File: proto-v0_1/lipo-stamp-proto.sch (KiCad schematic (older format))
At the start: 27 parts, among them Q1 Q_PMOS_GSD, U3 MCP73832-2-OT, U4 AP2112K-3.3, U5 AP9101CK6, U6 FS8205

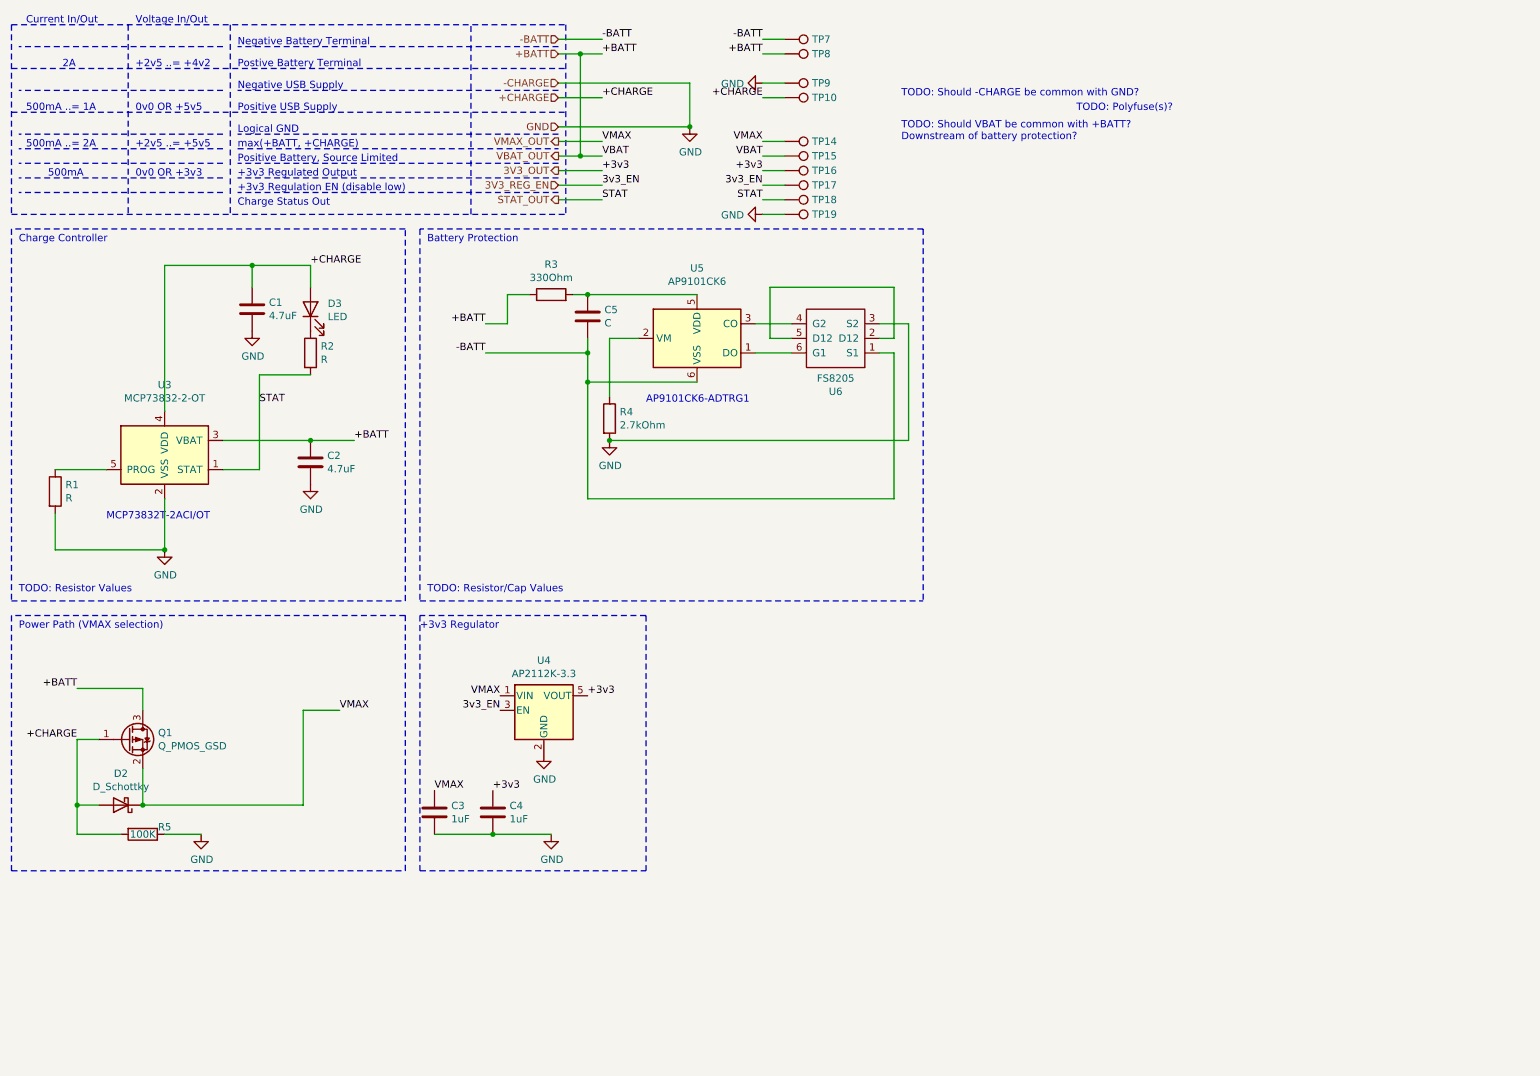
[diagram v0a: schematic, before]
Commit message: Going to start routing
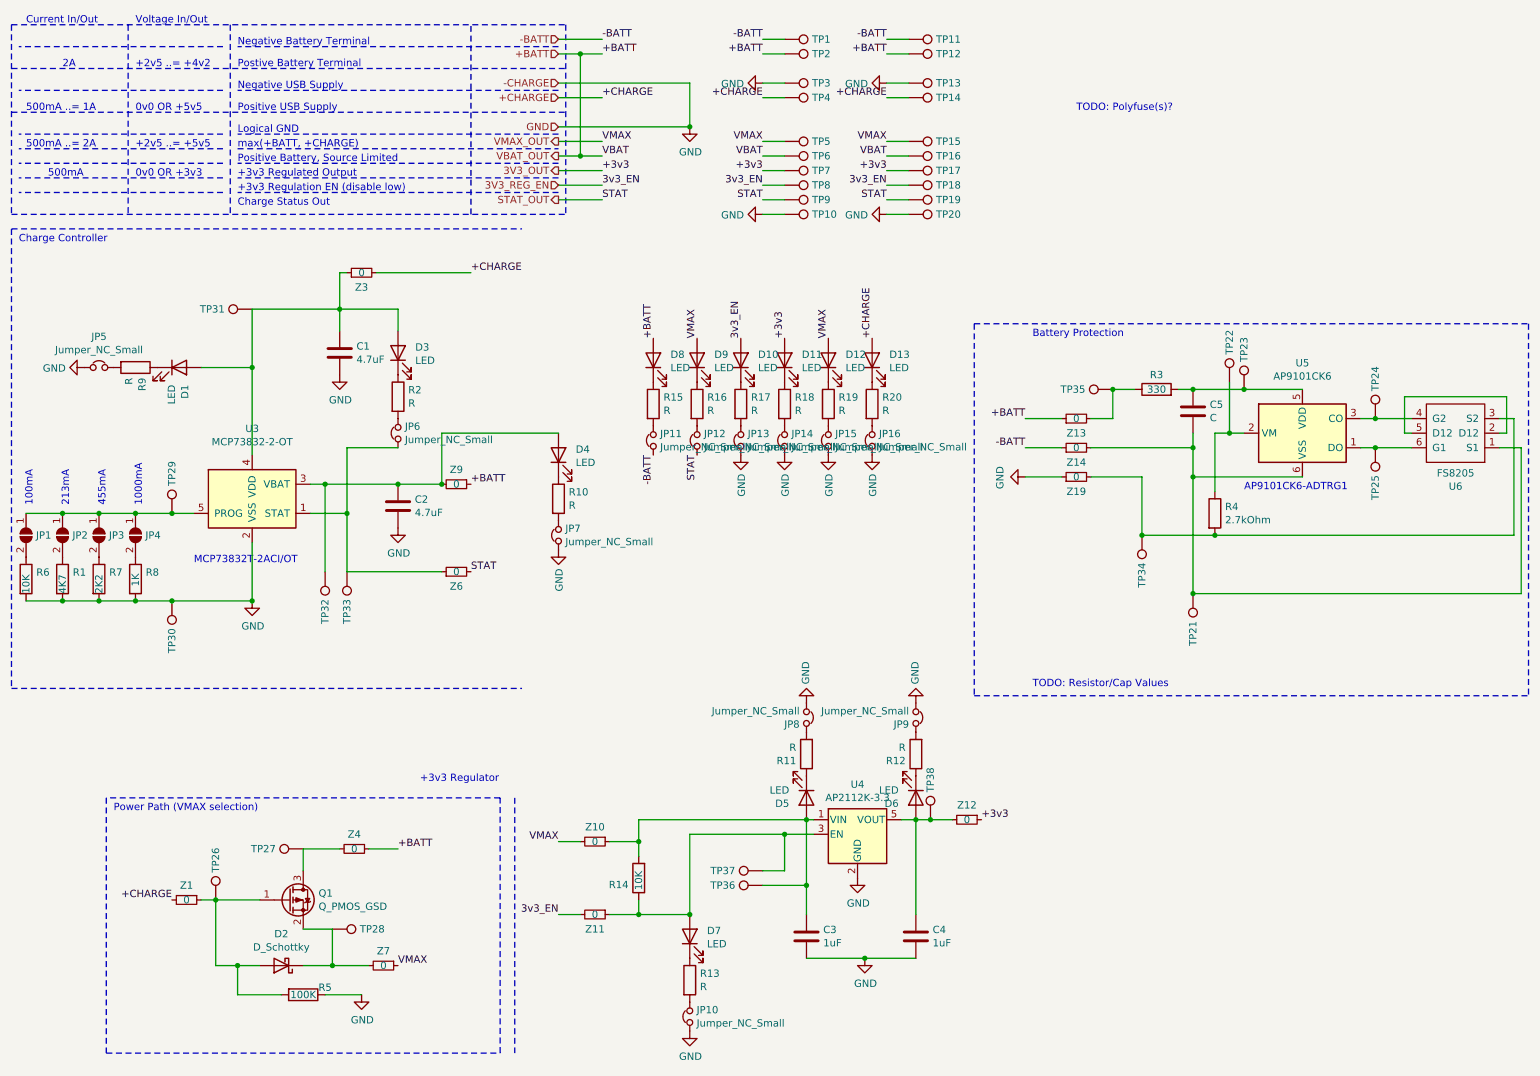
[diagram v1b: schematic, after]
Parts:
- added D1, D10, D11, D12, D13, D4, D5, D6, D7, D8, D9: LED, LED_SMD:LED_0805_2012Metric, symbol Device:LED
- added JP1, JP2, JP3, JP4: SolderJumper_2_Open, Jumper:SolderJumper-2_P1.3mm_Open_TrianglePad1.0x1.5mm, symbol Jumper:SolderJumper_2_Open
- added JP10, JP11, JP12, JP13, JP14, JP15, JP16, JP5, JP6, JP7, JP8, JP9: Jumper_NC_Small, Jumper:SolderJumper-2_P1.3mm_Bridged_RoundedPad1.0x1.5mm, symbol Device:Jumper_NC_Small
- added R10, R11, R12, R13, R15, R16, R17, R18, R19, R20, R9: R, Resistor_SMD:R_0805_2012Metric, symbol Device:R
- added R14, R6: 10K, Resistor_SMD:R_0805_2012Metric, symbol Device:R
- added R7: 2K2, Resistor_SMD:R_0805_2012Metric, symbol Device:R
- added R8: 1K, Resistor_SMD:R_0805_2012Metric, symbol Device:R
- added TP1, TP11, TP12, TP13, TP2, TP20, TP21, TP22, TP23, TP24, TP25, TP26, TP27, TP28, TP29, TP3, TP30, TP31, TP32, TP33, TP34, TP35, TP36, TP37, TP38, TP4, TP5, TP6: TestPoint, Everything:castellated-2-pin, symbol Connector:TestPoint
- added Z1, Z10, Z11, Z12, Z13, Z14, Z19, Z3, Z4, Z6, Z7, Z9: 0, Resistor_SMD:R_0805_2012Metric, symbol Device:R_Small
- R1: value R -> 4K7
- R3: value 330Ohm -> 330
- TP10, TP14, TP15, TP16, TP17, TP18, TP19, TP7, TP8, TP9: footprint Connector_PinHeader_2.54mm:PinHeader_1x01_P2.54mm_Vertical -> Everything:castellated-2-pin
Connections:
- net +BATT: now also TP16.1, D8.2 (A), TP12.1, TP2.1, TP6.1, Z13.1, Z4.1, Z9.1; no longer C2.1, Q1.3 (D), R3.1, TP15.1, TP8.1, U3.3 (VBAT)
- net +CHARGE: now also TP14.1, D13.2 (A), TP4.1, Z1.2, Z3.2; no longer C1.1, D2.2 (A), D3.2 (A), Q1.1 (G), R5.2, TP10.1, U3.4 (VDD)
- net -BATT: now also JP11.1, TP1.1, TP11.1, Z14.1; no longer C5.2, TP7.1, U5.6 (VSS), U6.1 (S1)
- net 3V3_OUT: now also TP17.1, TP7.1, D11.2 (A), Z12.1; no longer C4.1, TP16.1, U4.5 (VOUT)
- net 3V3_REG_EN: now also TP18.1, TP8.1, D10.2 (A), Z11.2; no longer TP17.1, U4.3 (EN)
- net GND: now also TP10.1, JP10.1, JP13.1, JP14.1, JP15.1, JP16.1, JP5.1, JP7.1, JP8.1, JP9.1, R6.2, R7.2, R8.2, TP13.1, TP20.1, TP3.1, TP30.1, Z19.1; no longer R4.2, TP19.1, TP9.1, U6.3 (S2)
- net STAT_OUT: now also TP19.1, TP9.1, JP12.1, Z6.2; no longer R2.2, TP18.1, U3.1 (STAT)
- net VMAX_OUT: now also TP15.1, D12.2 (A), D9.2 (A), TP5.1, Z10.2, Z7.1; no longer C3.1, D2.1 (K), Q1.2 (S), TP14.1, U4.1 (VIN)
- net at C5.1, R3.2, U5.5 (VDD): now also TP23.1
- net at R4.1, U5.2 (VM): now also TP22.1
- net at U3.5 (PROG): now also JP1.1 (A), JP2.1 (A), JP3.1 (A), JP4.1 (A), TP29.1; no longer R1.1
- net at U5.1 (DO), U6.6 (G1): now also TP25.1
- net at U5.3 (CO), U6.4 (G2): now also TP24.1
- new net: D2.1 (K), Q1.2 (S), TP28.1, Z7.2
- new net: D2.2 (A), Q1.1 (G), R5.2, TP26.1, Z1.1
- new net: Q1.3 (D), TP27.1, Z4.2
- new net: C3.1, D5.2 (A), R14.2, TP36.1, U4.1 (VIN), Z10.1
- new net: C4.1, D6.2 (A), TP38.1, U4.5 (VOUT), Z12.2
- new net: C5.2, TP21.1, U5.6 (VSS), U6.1 (S1), Z14.2
- new net: R4.2, TP34.1, U6.3 (S2), Z19.2
- new net: R3.1, TP35.1, Z13.2
- new net: C2.1, D4.2 (A), TP32.1, U3.3 (VBAT), Z9.2
- new net: C1.1, D1.2 (A), D3.2 (A), TP31.1, U3.4 (VDD), Z3.1
- new net: JP6.2, R2.2
- new net: JP6.1, TP33.1, U3.1 (STAT), Z6.1
- new net: JP2.2 (B), R1.1
- new net: D7.2 (A), R14.1, TP37.1, U4.3 (EN), Z11.1
- new net: JP1.2 (B), R6.1
- new net: JP4.2 (B), R8.1
- new net: JP3.2 (B), R7.1
- new net: D1.1 (K), R9.1
- new net: JP5.2, R9.2
- new net: D4.1 (K), R10.1
- new net: JP7.2, R10.2
- new net: D5.1 (K), R11.1
- new net: JP8.2, R11.2
- new net: D6.1 (K), R12.1
- new net: JP9.2, R12.2
- new net: D7.1 (K), R13.1
- new net: JP10.2, R13.2
- new net: D9.1 (K), R16.1
- new net: JP12.2, R16.2
- new net: D10.1 (K), R17.1
- new net: JP13.2, R17.2
- new net: D11.1 (K), R18.1
- new net: JP14.2, R18.2
- new net: D12.1 (K), R19.1
- new net: JP15.2, R19.2
- new net: D13.1 (K), R20.1
- new net: JP16.2, R20.2
- new net: D8.1 (K), R15.1
- new net: JP11.2, R15.2
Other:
- note added: "1000mA"
- note added: "100mA"
- note added: "213mA"
- note added: "455mA"
- note removed: "TODO: Resistor Values"
- note removed: "TODO: Should -CHARGE be common with GND?"
- note removed: "TODO: Should VBAT be common with +BATT?\nDownstream of battery protection?"
- moved on the sheet: C1, C2, C3, C4, C5, D2, D3, Q1, R1, R2, R3, R4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

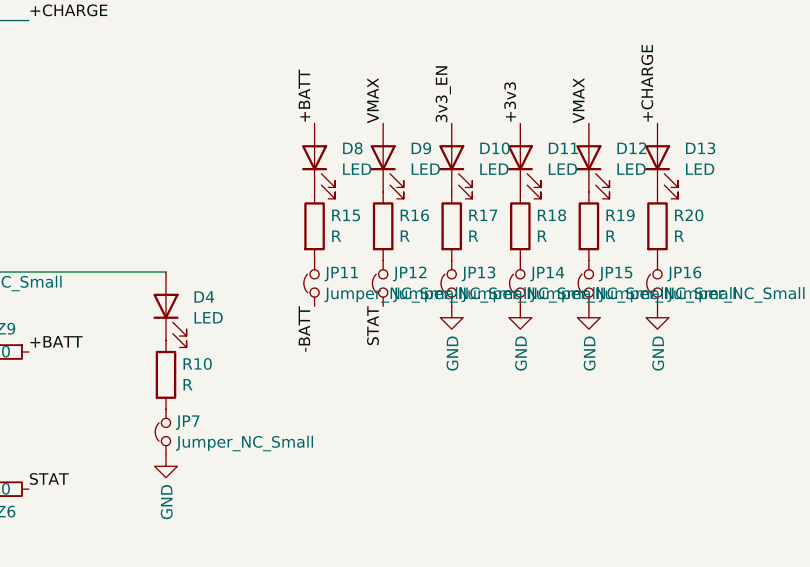
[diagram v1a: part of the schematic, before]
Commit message: Almost done, just needs back silkscreen
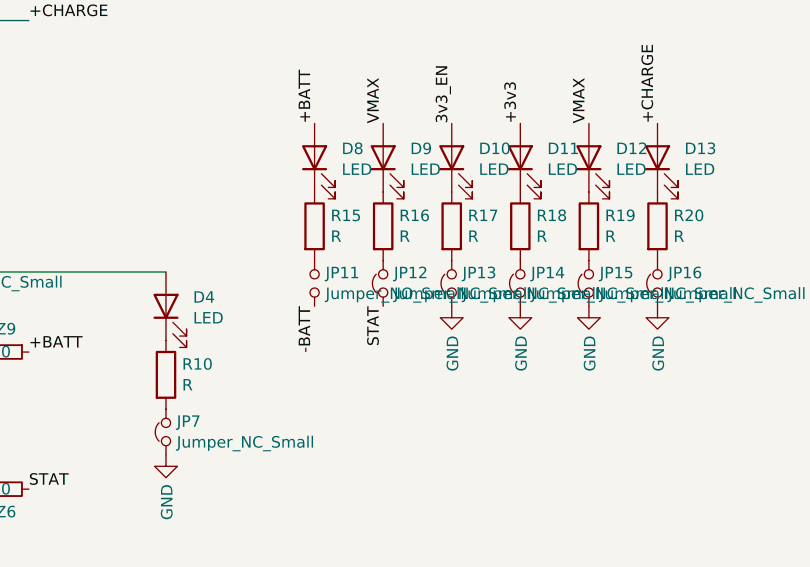
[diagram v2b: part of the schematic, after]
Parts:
- removed JP11: Jumper_NC_Small, Jumper:SolderJumper-2_P1.3mm_Bridged_RoundedPad1.0x1.5mm, symbol Device:Jumper_NC_Small
- added JP11: Jumper_NO_Small, Jumper:SolderJumper-2_P1.3mm_Open_RoundedPad1.0x1.5mm, symbol Device:Jumper_NO_Small
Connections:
- net -BATT: now also JP11.2
- net at R15.2: now also JP11.1
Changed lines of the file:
@@
 	1    0    0    -1
-$EndComp
-$Comp
-L Device:Jumper_NC_Small JP11
-U 1 1 604FB90A
-P 5000 3500
-F 0 "JP11" V 5046 3453 50  0000 R CNN
-F 1 "Jumper_NC_Small" V 4955 3453 50  0000 R CNN
-F 2 "Jumper:SolderJumper-2_P1.3mm_Bridged_RoundedPad1.0x1.5mm" H 5000 3500 50  0001 C CNN
-F 3 "~" H 5000 3500 50  0001 C CNN
-	1    5000 3500
-	0    -1   -1   0
 $EndComp
 Text Label 5000 2800 1    50   ~ 0
@@
 Text Label 5000 3600 3    50   ~ 0
 -BATT
+$Comp
+L Device:Jumper_NO_Small JP11
+U 1 1 6068AF95
+P 5000 3500
+F 0 "JP11" V 4954 3548 50  0000 L CNN
+F 1 "Jumper_NO_Small" V 5045 3548 50  0000 L CNN
+F 2 "Jumper:SolderJumper-2_P1.3mm_Open_RoundedPad1.0x1.5mm" H 5000 3500 50  0001 C CNN
+F 3 "~" H 5000 3500 50  0001 C CNN
+	1    5000 3500
+	0    1    1    0
+$EndComp
 $EndSCHEMATC
